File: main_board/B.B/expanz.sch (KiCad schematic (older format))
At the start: 23 parts, among them M1 Motor_DC, Q10 2N7002, Q7 SI3447CDV, Q8 2N7002, Q9 SI3447CDV, U68 IRM-H936, U70 MH253ESO, U71 MH253ESO

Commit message: uvolneni enkoderu
- dolomitelny enkoder
- zmenseni via u civek LDC
- vymena pouzdra USB-C
- otoceni IR prijmace
- zakas vylivani medi pod BMX9555
- odstraneni "ochrannych" odporu k M41T62
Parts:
- added J1, J4: Conn_01x04, Connector_PinSocket_2.54mm:PinSocket_1x04_P2.54mm_Vertical, symbol Connector_Generic:Conn_01x04
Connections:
- wire segments 35 -> 65

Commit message: popisky
-popisky
-poladeni uddeleni enkoderu
-poladeni nayvu drah
-priopjeni gnd USB
-poligon V5 na led-desce do spodni vrstvu
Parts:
- C114, C71, C72, C73, C74, C81: symbol Device:C -> B.B-rescue:C-Device
- D2: symbol Device:D -> B.B-rescue:D-Device
- D3: symbol Device:D_Schottky -> B.B-rescue:D_Schottky-Device
- J1, J4: symbol Connector_Generic:Conn_01x04 -> B.B-rescue:Conn_01x04-Connector_Generic
- M1: symbol Motor:Motor_DC -> B.B-rescue:Motor_DC-Motor
- Q10, Q8: symbol Transistor_FET:2N7002 -> B.B-rescue:2N7002-Transistor_FET
- R41, R42, R43, R46, R47, R5: symbol Device:R -> B.B-rescue:R-Device
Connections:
- wire segments 65 -> 69
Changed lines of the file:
@@
 EESchema Schematic File Version 4
-LIBS:B.B-cache
-EELAYER 29 0
+EELAYER 30 0
 EELAYER END
 $Descr A4 11693 8268
 encoding utf-8
-Sheet 6 8
+Sheet 5 8
 Title ""
 Date ""
@@
 $EndDescr
 $Comp
-L Motor:Motor_DC M1
+L B.B-rescue:Motor_DC-Motor M1
 U 1 1 5FA5194A
 P 4825 4500
@@
 MOTOR
 $Comp
-L Device:R R?
+L B.B-rescue:R-Device R?
 U 1 1 5FAA51EC
 P 3425 4550
@@
 	3225 4250 3425 4250
 $Comp
-L Device:D_Schottky D?
+L B.B-rescue:D_Schottky-Device D?
 U 1 1 5FBB2FF1
 P 4525 4600
@@
 5V
 $Comp
-L Device:R R?
+L B.B-rescue:R-Device R?
 U 1 1 5FAAB362
 P 7550 2525
@@
 	8950 4700 9350 4700
 $Comp
-L Device:C C?
+L B.B-rescue:C-Device C?
 U 1 1 5FB5B58D
 P 10100 4900
@@
 $EndComp
 $Comp
-L Device:R R?
+L B.B-rescue:R-Device R?
 U 1 1 5FB5B594
 P 10100 4500
@@
 3V3
 $Comp
-L Device:C C?
+L B.B-rescue:C-Device C?
 U 1 1 5FB5B5B5
 P 6900 4900
@@
 	6900 4700 7300 4700
 $Comp
-L Device:C C?
+L B.B-rescue:C-Device C?
 U 1 1 5FB5B5C6
 P 8050 4900
@@
 $EndComp
 $Comp
-L Device:R R?
+L B.B-rescue:R-Device R?
 U 1 1 5FB5B5CD
 P 8050 4500
@@
 Connection ~ 8050 4700
 $Comp
-L Device:C C?
+L B.B-rescue:C-Device C?
 U 1 1 5FB5B5DB
 P 8950 4900
@@
 $EndComp
 $Comp
-L Transistor_FET:2N7002 Q?
+L B.B-rescue:2N7002-Transistor_FET Q?
 U 1 1 5FBA8934
 P 7650 2725
@@
 Connection ~ 7750 2525
 $Comp
-L Transistor_FET:2N7002 Q?
+L B.B-rescue:2N7002-Transistor_FET Q?
 U 1 1 5FBAB051
 P 3525 4750
@@
 	1    0    0    -1
 $EndComp
-Text HLabel 5350 2200 1    50   Input ~ 0
-IR-OUT
-$Comp
-L B.B-eagle-import:LED LED?
-U 1 1 5FA465E8
-P 5350 2600
-AR Path="/5FA3274C/5FA465E8" Ref="LED?"  Part="1"
-AR Path="/5F9EE529/5FA465E8" Ref="LED3"  Part="1"
-F 0 "LED3" H 5428 2603 59  0000 L CNN
-F 1 "IR" H 5428 2498 59  0000 L CNN
-F 2 "LED_SMD:LED_0603_1608Metric" H 5350 2600 50  0001 C CNN
-F 3 "" H 5350 2600 50  0001 C CNN
-F 4 "C142316" H 5350 2600 50  0001 C CNN "LCSC"
-	1    5350 2600
-	1    0    0    -1
-$EndComp
-$Comp
-L B.B-eagle-import:GND #GND?
-U 1 1 5FA465EE
-P 5350 2900
-AR Path="/5FA3274C/5FA465EE" Ref="#GND?"  Part="1"
-AR Path="/5F9EE529/5FA465EE" Ref="#GND0140"  Part="1"
-F 0 "#GND0140" H 5350 2900 50  0001 C CNN
-F 1 "GND" H 5350 2820 59  0000 C CNN
-F 2 "" H 5350 2900 50  0001 C CNN
-F 3 "" H 5350 2900 50  0001 C CNN
-	1    5350 2900
-	1    0    0    -1
-$EndComp
 $Comp
 L B.B-rescue:IRM-H936 U?
@@
 $EndComp
 $Comp
-L Device:C C?
+L B.B-rescue:C-Device C?
 U 1 1 5FB0693F
 P 3375 2650
@@
 	3375 2450 3850 2450
 $Comp
-L Device:R R?
-U 1 1 5FA5476F
-P 5350 2350
-AR Path="/5FA3274C/5FA5476F" Ref="R?"  Part="1"
-AR Path="/5F9EE529/5FA5476F" Ref="R43"  Part="1"
-F 0 "R43" V 5143 2350 50  0000 C CNN
-F 1 "220" V 5234 2350 50  0000 C CNN
-F 2 "Resistor_SMD:R_0402_1005Metric" V 5280 2350 50  0001 C CNN
-F 3 "~" H 5350 2350 50  0001 C CNN
-F 4 "C25092" V 5350 2350 50  0001 C CNN "LCSC"
-	1    5350 2350
-	-1   0    0    1
-$EndComp
-$Comp
 L B.B-rescue:Q_PMOS_DSG Q7
 U 1 1 5FBE7385
@@
 VCC
 $Comp
-L Device:D D?
+L B.B-rescue:D-Device D?
 U 1 1 5FCDB883
 P 2875 2450
@@
 $EndComp
 $Comp
-L Device:C C?
+L B.B-rescue:C-Device C?
 U 1 1 5FCDDF04
 P 3850 2650
@@
 $EndComp
 $Comp
-L Device:R R?
+L B.B-rescue:R-Device R?
 U 1 1 5FD86664
 P 3175 2450
@@
 $EndComp
 $Comp
-L Connector_Generic:Conn_01x04 J1
+L B.B-rescue:Conn_01x04-Connector_Generic J1
 U 1 1 5FE739E9
 P 6100 4700
+AR Path="/5FE739E9" Ref="J1"  Part="1"
+AR Path="/5F9EE529/5FE739E9" Ref="J1"  Part="1"
 F 0 "J1" H 6050 4900 50  0000 L CNN
 F 1 "Conn_01x04" V 6200 4400 50  0000 L CNN
@@
 Connection ~ 8950 5100
 Wire Wire Line
-	8950 5100 8050 5100
-Wire Wire Line
 	6900 4700 6900 4300
 Wire Wire Line
@@
 	8050 4350 8050 4300
 Connection ~ 8050 4300
-Wire Wire Line
-	8050 4300 8950 4300
 $Comp
 L B.B-eagle-import:GND #GND0114
@@
 	10100 4700 10350 4700
 $Comp
-L Connector_Generic:Conn_01x04 J4
+L B.B-rescue:Conn_01x04-Connector_Generic J4
 U 1 1 5FE71BD6
 P 6300 4700
+AR Path="/5FE71BD6" Ref="J4"  Part="1"
+AR Path="/5F9EE529/5FE71BD6" Ref="J4"  Part="1"
 F 0 "J4" H 6300 4400 50  0000 C CNN
 F 1 "Conn_01x04" V 6400 4625 50  0000 C CNN
@@
 	-1   0    0    1
 $EndComp
+Wire Wire Line
+	5900 4800 6500 4800
+Connection ~ 5900 4800
+Connection ~ 6500 4800
+Wire Wire Line
+	6500 4700 5900 4700
+Connection ~ 6500 4700
+Wire Wire Line
+	5900 4600 6500 4600
+Connection ~ 6500 4600
+Wire Wire Line
+	6500 4500 5900 4500
+Connection ~ 6500 4500
+$Comp
+L B.B-rescue:R-Device R?
+U 1 1 5FA5476F
+P 5350 2350
+AR Path="/5FA3274C/5FA5476F" Ref="R?"  Part="1"
+AR Path="/5F9EE529/5FA5476F" Ref="R43"  Part="1"
+F 0 "R43" V 5143 2350 50  0000 C CNN
+F 1 "220" V 5234 2350 50  0000 C CNN
+F 2 "Resistor_SMD:R_0402_1005Metric" V 5280 2350 50  0001 C CNN
+F 3 "~" H 5350 2350 50  0001 C CNN
+F 4 "C25092" V 5350 2350 50  0001 C CNN "LCSC"
+	1    5350 2350
+	-1   0    0    1
+$EndComp
+$Comp
+L B.B-eagle-import:GND #GND?
+U 1 1 5FA465EE
+P 5350 2900
+AR Path="/5FA3274C/5FA465EE" Ref="#GND?"  Part="1"
+AR Path="/5F9EE529/5FA465EE" Ref="#GND0140"  Part="1"
+F 0 "#GND0140" H 5350 2900 50  0001 C CNN
+F 1 "GND" H 5350 2820 59  0000 C CNN
+F 2 "" H 5350 2900 50  0001 C CNN
+F 3 "" H 5350 2900 50  0001 C CNN
+	1    5350 2900
+	1    0    0    -1
+$EndComp
+$Comp
+L B.B-eagle-import:LED LED?
+U 1 1 5FA465E8
+P 5350 2600
+AR Path="/5FA3274C/5FA465E8" Ref="LED?"  Part="1"
+AR Path="/5F9EE529/5FA465E8" Ref="LED3"  Part="1"
+F 0 "LED3" H 5428 2603 59  0000 L CNN
+F 1 "IR" H 5428 2498 59  0000 L CNN
+F 2 "LED_SMD:LED_0603_1608Metric" H 5350 2600 50  0001 C CNN
+F 3 "" H 5350 2600 50  0001 C CNN
+F 4 "C142316" H 5350 2600 50  0001 C CNN "LCSC"
+	1    5350 2600
+	1    0    0    -1
+$EndComp
+Text HLabel 5350 2200 1    50   Input ~ 0
+IR-OUT
+Wire Wire Line
+	8050 5100 8950 5100
+Wire Wire Line
+	8050 4300 8950 4300
 $EndSCHEMATC

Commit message: LDC footprint
prodlouzeni pedu pro usnadneni rucniho osazovani
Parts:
- C114, C71, C72, C73, C74, C81: symbol B.B-rescue:C-Device -> B.B-rescue:C-Device-B.B-rescue
- D2: symbol B.B-rescue:D-Device -> B.B-rescue:D-Device-B.B-rescue
- D3: symbol B.B-rescue:D_Schottky-Device -> B.B-rescue:D_Schottky-Device-B.B-rescue
- J1, J4: symbol B.B-rescue:Conn_01x04-Connector_Generic -> B.B-rescue:Conn_01x04-Connector_Generic-B.B-rescue
- LED3: symbol B.B-eagle-import:LED -> B.B-rescue:LED-B.B-eagle-import
- M1: symbol B.B-rescue:Motor_DC-Motor -> B.B-rescue:Motor_DC-Motor-B.B-rescue
- Q10, Q8: symbol B.B-rescue:2N7002-Transistor_FET -> B.B-rescue:2N7002-Transistor_FET-B.B-rescue
- Q7, Q9: symbol B.B-rescue:Q_PMOS_DSG -> B.B-rescue:Q_PMOS_DSG-B.B-rescue
- R41, R42, R43, R46, R47, R5: symbol B.B-rescue:R-Device -> B.B-rescue:R-Device-B.B-rescue
- U68: symbol B.B-rescue:IRM-H936 -> B.B-rescue:IRM-H936-B.B-rescue
- U70, U71: symbol B.B-rescue:MH253ESO -> B.B-rescue:MH253ESO-B.B-rescue; LCSC (none) -> C114369
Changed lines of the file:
@@
 $EndDescr
 $Comp
-L B.B-rescue:Motor_DC-Motor M1
+L B.B-rescue:Motor_DC-Motor-B.B-rescue M1
 U 1 1 5FA5194A
 P 4825 4500
@@
 	4825 4800 4825 4950
 $Comp
-L B.B-eagle-import:GND #GND0132
+L B.B-rescue:GND-B.B-eagle-import #GND0132
 U 1 1 5FA5FD95
 P 3625 5050
@@
 $EndComp
 $Comp
-L B.B-eagle-import:GND #GND0134
+L B.B-rescue:GND-B.B-eagle-import #GND0134
 U 1 1 5FA60281
 P 5850 4950
@@
 $EndComp
 $Comp
-L B.B-eagle-import:GND #GND0133
+L B.B-rescue:GND-B.B-eagle-import #GND0133
 U 1 1 5FAF4CA6
 P 4525 5050
@@
 MOTOR
 $Comp
-L B.B-rescue:R-Device R?
+L B.B-rescue:R-Device-B.B-rescue R?
 U 1 1 5FAA51EC
 P 3425 4550
@@
 	3225 4250 3425 4250
 $Comp
-L B.B-rescue:D_Schottky-Device D?
+L B.B-rescue:D_Schottky-Device-B.B-rescue D?
 U 1 1 5FBB2FF1
 P 4525 4600
@@
 $EndComp
 $Comp
-L B.B-eagle-import:GND #GND0137
+L B.B-rescue:GND-B.B-eagle-import #GND0137
 U 1 1 5F9DF814
 P 7750 3025
@@
 5V
 $Comp
-L B.B-rescue:R-Device R?
+L B.B-rescue:R-Device-B.B-rescue R?
 U 1 1 5FAAB362
 P 7550 2525
@@
 WS2812-power
 $Comp
-L B.B-rescue:MH253ESO U?
+L B.B-rescue:MH253ESO-B.B-rescue U?
 U 1 1 5FB5B56F
 P 9650 4700
@@
 F 2 "Package_TO_SOT_SMD:SOT-23" H 9650 4750 50  0001 C CNN
 F 3 "https://datasheet.lcsc.com/szlcsc/Magnesensor-Tech-MST-MH253ESO_C114369.pdf" H 9650 4750 50  0001 C CNN
+F 4 "C114369" H 9650 4700 50  0001 C CNN "LCSC"
 	1    9650 4700
 	1    0    0    -1
@@
 	8950 4700 9350 4700
 $Comp
-L B.B-rescue:C-Device C?
+L B.B-rescue:C-Device-B.B-rescue C?
 U 1 1 5FB5B58D
 P 10100 4900
@@
 $EndComp
 $Comp
-L B.B-rescue:R-Device R?
+L B.B-rescue:R-Device-B.B-rescue R?
 U 1 1 5FB5B594
 P 10100 4500
@@
 Connection ~ 10100 4700
 $Comp
-L B.B-rescue:MH253ESO U?
+L B.B-rescue:MH253ESO-B.B-rescue U?
 U 1 1 5FB5B5A1
 P 7600 4700
@@
 F 2 "Package_TO_SOT_SMD:SOT-23" H 7600 4750 50  0001 C CNN
 F 3 "https://datasheet.lcsc.com/szlcsc/Magnesensor-Tech-MST-MH253ESO_C114369.pdf" H 7600 4750 50  0001 C CNN
+F 4 "C114369" H 7600 4700 50  0001 C CNN "LCSC"
 	1    7600 4700
 	1    0    0    -1
@@
 3V3
 $Comp
-L B.B-rescue:C-Device C?
+L B.B-rescue:C-Device-B.B-rescue C?
 U 1 1 5FB5B5B5
 P 6900 4900
@@
 	6900 4700 7300 4700
 $Comp
-L B.B-rescue:C-Device C?
+L B.B-rescue:C-Device-B.B-rescue C?
 U 1 1 5FB5B5C6
 P 8050 4900
@@
 $EndComp
 $Comp
-L B.B-rescue:R-Device R?
+L B.B-rescue:R-Device-B.B-rescue R?
 U 1 1 5FB5B5CD
 P 8050 4500
@@
 Connection ~ 8050 4700
 $Comp
-L B.B-rescue:C-Device C?
+L B.B-rescue:C-Device-B.B-rescue C?
 U 1 1 5FB5B5DB
 P 8950 4900
@@
 $EndComp
 $Comp
-L B.B-rescue:Q_PMOS_DSG Q9
+L B.B-rescue:Q_PMOS_DSG-B.B-rescue Q9
 U 1 1 602B1909
 P 7750 2325
@@
 $EndComp
 $Comp
-L B.B-rescue:2N7002-Transistor_FET Q?
+L B.B-rescue:2N7002-Transistor_FET-B.B-rescue Q?
 U 1 1 5FBA8934
 P 7650 2725
@@
 Connection ~ 7750 2525
 $Comp
-L B.B-rescue:2N7002-Transistor_FET Q?
+L B.B-rescue:2N7002-Transistor_FET-B.B-rescue Q?
 U 1 1 5FBAB051
 P 3525 4750
@@
 Connection ~ 3625 4550
 $Comp
-L B.B-eagle-import:GND #GND?
+L B.B-rescue:GND-B.B-eagle-import #GND?
 U 1 1 5FA465E0
 P 4350 2900
@@
 $EndComp
 $Comp
-L B.B-rescue:IRM-H936 U?
+L B.B-rescue:IRM-H936-B.B-rescue U?
 U 1 1 5FA465F6
 P 4350 2450
@@
 $EndComp
 $Comp
-L B.B-rescue:C-Device C?
+L B.B-rescue:C-Device-B.B-rescue C?
 U 1 1 5FB0693F
 P 3375 2650
@@
 $EndComp
 $Comp
-L B.B-eagle-import:GND #GND?
+L B.B-rescue:GND-B.B-eagle-import #GND?
 U 1 1 5FB06945
 P 3375 2900
@@
 	3375 2450 3850 2450
 $Comp
-L B.B-rescue:Q_PMOS_DSG Q7
+L B.B-rescue:Q_PMOS_DSG-B.B-rescue Q7
 U 1 1 5FBE7385
 P 3625 4350
@@
 VCC
 $Comp
-L B.B-rescue:D-Device D?
+L B.B-rescue:D-Device-B.B-rescue D?
 U 1 1 5FCDB883
 P 2875 2450
@@
 $EndComp
 $Comp
-L B.B-rescue:C-Device C?
+L B.B-rescue:C-Device-B.B-rescue C?
 U 1 1 5FCDDF04
 P 3850 2650
@@
 	3850 2450 4050 2450
 $Comp
-L B.B-eagle-import:GND #GND?
+L B.B-rescue:GND-B.B-eagle-import #GND?
 U 1 1 5FCE1B74
 P 3850 2900
@@
 $EndComp
 $Comp
-L B.B-rescue:R-Device R?
+L B.B-rescue:R-Device-B.B-rescue R?
 U 1 1 5FD86664
 P 3175 2450
@@
 $EndComp
 $Comp
-L B.B-rescue:Conn_01x04-Connector_Generic J1
+L B.B-rescue:Conn_01x04-Connector_Generic-B.B-rescue J1
 U 1 1 5FE739E9
 P 6100 4700
@@
 Connection ~ 8050 4300
 $Comp
-L B.B-eagle-import:GND #GND0114
+L B.B-rescue:GND-B.B-eagle-import #GND0114
 U 1 1 5FE93EA1
 P 4825 5050
@@
 	10100 4700 10350 4700
 $Comp
-L B.B-rescue:Conn_01x04-Connector_Generic J4
+L B.B-rescue:Conn_01x04-Connector_Generic-B.B-rescue J4
 U 1 1 5FE71BD6
 P 6300 4700
@@
 Connection ~ 6500 4500
 $Comp
-L B.B-rescue:R-Device R?
+L B.B-rescue:R-Device-B.B-rescue R?
 U 1 1 5FA5476F
 P 5350 2350
@@
 $EndComp
 $Comp
-L B.B-eagle-import:GND #GND?
+L B.B-rescue:GND-B.B-eagle-import #GND?
 U 1 1 5FA465EE
 P 5350 2900
@@
 $EndComp
 $Comp
-L B.B-eagle-import:LED LED?
+L B.B-rescue:LED-B.B-eagle-import LED?
 U 1 1 5FA465E8
 P 5350 2600

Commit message: JLCdata
- korekce pozice a natoceni
- data pro vyrobu
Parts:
- Q10, Q8, U70, U71: JLCPCB_CORRECTION (none) -> 0;0;180
- Q7, Q9: LCSC C145421 -> C144884
- U68: JLCPCB_CORRECTION (none) -> 0;0.88;0
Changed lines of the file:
@@
 $Descr A4 11693 8268
 encoding utf-8
-Sheet 5 8
+Sheet 8 8
 Title ""
 Date ""
@@
 F 3 "https://datasheet.lcsc.com/szlcsc/Magnesensor-Tech-MST-MH253ESO_C114369.pdf" H 9650 4750 50  0001 C CNN
 F 4 "C114369" H 9650 4700 50  0001 C CNN "LCSC"
+F 5 "0;0;180" H 9650 4700 50  0001 C CNN "JLCPCB_CORRECTION"
 	1    9650 4700
 	1    0    0    -1
@@
 F 3 "https://datasheet.lcsc.com/szlcsc/Magnesensor-Tech-MST-MH253ESO_C114369.pdf" H 7600 4750 50  0001 C CNN
 F 4 "C114369" H 7600 4700 50  0001 C CNN "LCSC"
+F 5 "0;0;180" H 7600 4700 50  0001 C CNN "JLCPCB_CORRECTION"
 	1    7600 4700
 	1    0    0    -1
@@
 F 2 "BB:TSOP-6_1.5x3.0x0.95P" H 7950 2425 50  0001 C CNN
 F 3 "https://datasheet.lcsc.com/szlcsc/Vishay-Intertech-SI3447CDV-T1-E3_C145421.pdf" H 7750 2325 50  0001 C CNN
-F 4 "C145421" V 7750 2325 50  0001 C CNN "LCSC"
+F 4 "C144884" V 7750 2325 50  0001 C CNN "LCSC"
 	1    7750 2325
 	0    1    -1   0
@@
 F 3 "https://datasheet.lcsc.com/szlcsc/Changjiang-Electronics-Tech-CJ-CJ3134K_C110100.pdf" H 7650 2725 50  0001 L CNN
 F 4 "C8545" H 7650 2725 50  0001 C CNN "LCSC"
+F 5 "0;0;180" H 7650 2725 50  0001 C CNN "JLCPCB_CORRECTION"
 	1    7650 2725
 	1    0    0    -1
@@
 F 3 "https://datasheet.lcsc.com/szlcsc/Changjiang-Electronics-Tech-CJ-CJ3134K_C110100.pdf" H 3525 4750 50  0001 L CNN
 F 4 "C8545" H 3525 4750 50  0001 C CNN "LCSC"
+F 5 "0;0;180" H 3525 4750 50  0001 C CNN "JLCPCB_CORRECTION"
 	1    3525 4750
 	1    0    0    -1
@@
 F 3 "" H 4350 2900 50  0001 C CNN
 	1    4350 2900
-	1    0    0    -1
-$EndComp
-$Comp
-L B.B-rescue:IRM-H936-B.B-rescue U?
-U 1 1 5FA465F6
-P 4350 2450
-AR Path="/5FA3274C/5FA465F6" Ref="U?"  Part="1"
-AR Path="/5F9EE529/5FA465F6" Ref="U68"  Part="1"
-F 0 "U68" H 4350 2675 50  0000 C CNN
-F 1 "IRM-H936" H 4350 2584 50  0000 C CNN
-F 2 "BB:SMD-4_4.0x5.0x2.54P" H 4350 2450 50  0001 C CNN
-F 3 "https://datasheet.lcsc.com/szlcsc/1912111437_Everlight-Elec-IRM-H936-TR2_C264266.pdf" H 4350 2450 50  0001 C CNN
-F 4 "C264266" H 4350 2450 50  0001 C CNN "LCSC"
-	1    4350 2450
 	1    0    0    -1
 $EndComp
@@
 F 2 "BB:TSOP-6_1.5x3.0x0.95P" H 3825 4450 50  0001 C CNN
 F 3 "https://datasheet.lcsc.com/szlcsc/Vishay-Intertech-SI3447CDV-T1-E3_C145421.pdf" H 3625 4350 50  0001 C CNN
-F 4 "C145421" V 3625 4350 50  0001 C CNN "LCSC"
+F 4 "C144884" V 3625 4350 50  0001 C CNN "LCSC"
 	1    3625 4350
 	0    1    -1   0
@@
 Wire Wire Line
 	8050 4300 8950 4300
+$Comp
+L B.B-rescue:IRM-H936-B.B-rescue U?
+U 1 1 5FA465F6
+P 4350 2450
+AR Path="/5FA3274C/5FA465F6" Ref="U?"  Part="1"
+AR Path="/5F9EE529/5FA465F6" Ref="U68"  Part="1"
+F 0 "U68" H 4350 2675 50  0000 C CNN
+F 1 "IRM-H936" H 4350 2584 50  0000 C CNN
+F 2 "BB:SMD-4_4.0x5.0x2.54P" H 4350 2450 50  0001 C CNN
+F 3 "https://datasheet.lcsc.com/szlcsc/1912111437_Everlight-Elec-IRM-H936-TR2_C264266.pdf" H 4350 2450 50  0001 C CNN
+F 4 "C264266" H 4350 2450 50  0001 C CNN "LCSC"
+F 5 "0;0.88;0" H 4350 2450 50  0001 C CNN "JLCPCB_CORRECTION"
+	1    4350 2450
+	1    0    0    -1
+$EndComp
 $EndSCHEMATC

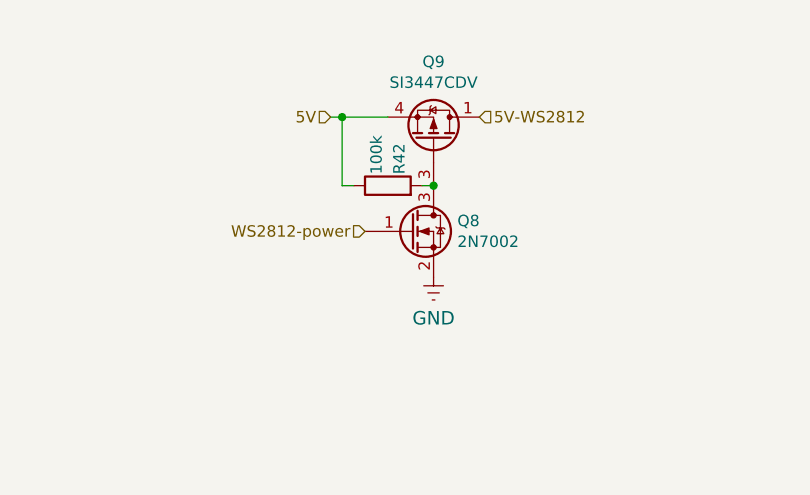
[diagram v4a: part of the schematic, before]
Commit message: opravi_a_dodatky MPU/QMC/conn_A9G
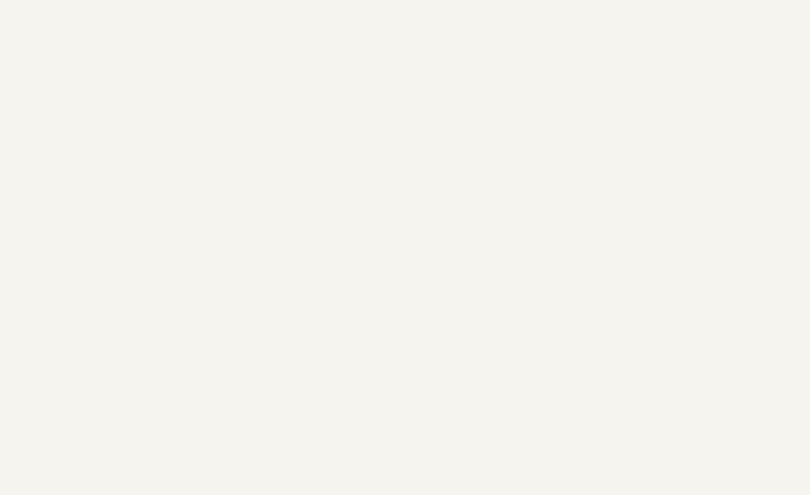
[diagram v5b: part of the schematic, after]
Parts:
- removed Q8: 2N7002, Package_TO_SOT_SMD:SOT-23, symbol B.B-rescue:2N7002-Transistor_FET-B.B-rescue
- removed Q9: SI3447CDV, BB:TSOP-6_1.5x3.0x0.95P, symbol B.B-rescue:Q_PMOS_DSG-B.B-rescue
- removed R42: 100k, Resistor_SMD:R_0402_1005Metric, symbol B.B-rescue:R-Device-B.B-rescue
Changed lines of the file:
@@
 EESchema Schematic File Version 4
-EELAYER 30 0
+LIBS:B.B-cache
+EELAYER 29 0
 EELAYER END
 $Descr A4 11693 8268
 encoding utf-8
-Sheet 8 8
+Sheet 7 8
 Title ""
 Date ""
@@
 $EndComp
 $Comp
-L B.B-rescue:GND-B.B-eagle-import #GND0137
-U 1 1 5F9DF814
-P 7750 3025
-AR Path="/5F9EE529/5F9DF814" Ref="#GND0137"  Part="1"
-AR Path="/5FA9DBB3/5F9DF814" Ref="#GND?"  Part="1"
-F 0 "#GND0137" H 7750 3025 50  0001 C CNN
-F 1 "GND" H 7750 2945 59  0000 C CNN
-F 2 "" H 7750 3025 50  0001 C CNN
-F 3 "" H 7750 3025 50  0001 C CNN
-	1    7750 3025
-	1    0    0    -1
-$EndComp
-Text HLabel 7950 2225 2    50   Input ~ 0
-5V-WS2812
-Text HLabel 7300 2225 0    50   Input ~ 0
-5V
-$Comp
-L B.B-rescue:R-Device-B.B-rescue R?
-U 1 1 5FAAB362
-P 7550 2525
-AR Path="/5F96CFDA/5FAAB362" Ref="R?"  Part="1"
-AR Path="/5F9EE529/5F9F24D4/5FAAB362" Ref="R?"  Part="1"
-AR Path="/5FA9DBB3/5F9F24D4/5FAAB362" Ref="R?"  Part="1"
-AR Path="/5F9EE529/5FAAB362" Ref="R42"  Part="1"
-F 0 "R42" H 7600 2475 50  0000 L CNN
-F 1 "100k" H 7600 2575 50  0000 L CNN
-F 2 "Resistor_SMD:R_0402_1005Metric" V 7480 2525 50  0001 C CNN
-F 3 "~" H 7550 2525 50  0001 C CNN
-F 4 "C25741" H 7550 2525 50  0001 C CNN "LCSC"
-	1    7550 2525
-	0    -1   -1   0
-$EndComp
-Wire Wire Line
-	7700 2525 7750 2525
-Wire Wire Line
-	7300 2225 7350 2225
-Wire Wire Line
-	7400 2525 7350 2525
-Wire Wire Line
-	7350 2525 7350 2225
-Connection ~ 7350 2225
-Wire Wire Line
-	7350 2225 7550 2225
-Text HLabel 7450 2725 0    50   Input ~ 0
-WS2812-power
-$Comp
 L B.B-rescue:MH253ESO-B.B-rescue U?
 U 1 1 5FB5B56F
@@
 $EndComp
 $Comp
-L B.B-rescue:Q_PMOS_DSG-B.B-rescue Q9
-U 1 1 602B1909
-P 7750 2325
-F 0 "Q9" V 8092 2325 50  0000 C CNN
-F 1 "SI3447CDV" V 8001 2325 50  0000 C CNN
-F 2 "BB:TSOP-6_1.5x3.0x0.95P" H 7950 2425 50  0001 C CNN
-F 3 "https://datasheet.lcsc.com/szlcsc/Vishay-Intertech-SI3447CDV-T1-E3_C145421.pdf" H 7750 2325 50  0001 C CNN
-F 4 "C144884" V 7750 2325 50  0001 C CNN "LCSC"
-	1    7750 2325
-	0    1    -1   0
-$EndComp
-$Comp
 L B.B-rescue:2N7002-Transistor_FET-B.B-rescue Q?
-U 1 1 5FBA8934
-P 7650 2725
-AR Path="/5F77B818/5FBA8934" Ref="Q?"  Part="1"
-AR Path="/5FA4C94D/5FBA8934" Ref="Q?"  Part="1"
-AR Path="/5F9EE529/5FBA8934" Ref="Q8"  Part="1"
-F 0 "Q8" H 7854 2771 50  0000 L CNN
-F 1 "2N7002" H 7854 2680 50  0000 L CNN
-F 2 "Package_TO_SOT_SMD:SOT-23" H 7850 2650 50  0001 L CIN
-F 3 "https://datasheet.lcsc.com/szlcsc/Changjiang-Electronics-Tech-CJ-CJ3134K_C110100.pdf" H 7650 2725 50  0001 L CNN
-F 4 "C8545" H 7650 2725 50  0001 C CNN "LCSC"
-F 5 "0;0;180" H 7650 2725 50  0001 C CNN "JLCPCB_CORRECTION"
-	1    7650 2725
-	1    0    0    -1
-$EndComp
-Connection ~ 7750 2525
-$Comp
-L B.B-rescue:2N7002-Transistor_FET-B.B-rescue Q?
